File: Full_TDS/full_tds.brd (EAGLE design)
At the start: 69.5 x 52.1 mm, 66 parts, among them IC1 MCP1702, Q5 8MHz, SW1 MAIN, SW2 PI, SW3 SENSOR, U2 FT232RLSSOP, U3 ADXL345PATRICK, U4 MPL3115A2LGA8, U5 ATMEGA328P_TQFP

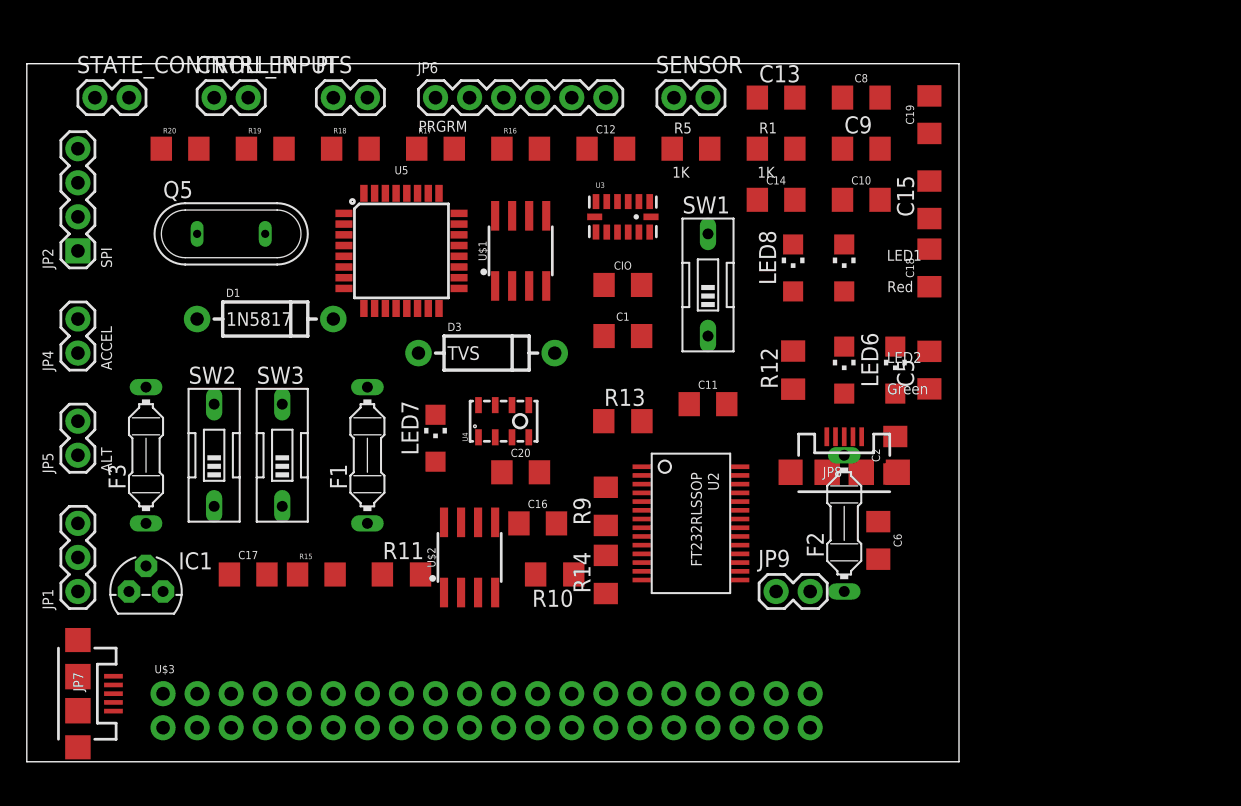
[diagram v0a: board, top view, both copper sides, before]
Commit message: Some schematic adjustments and board progress
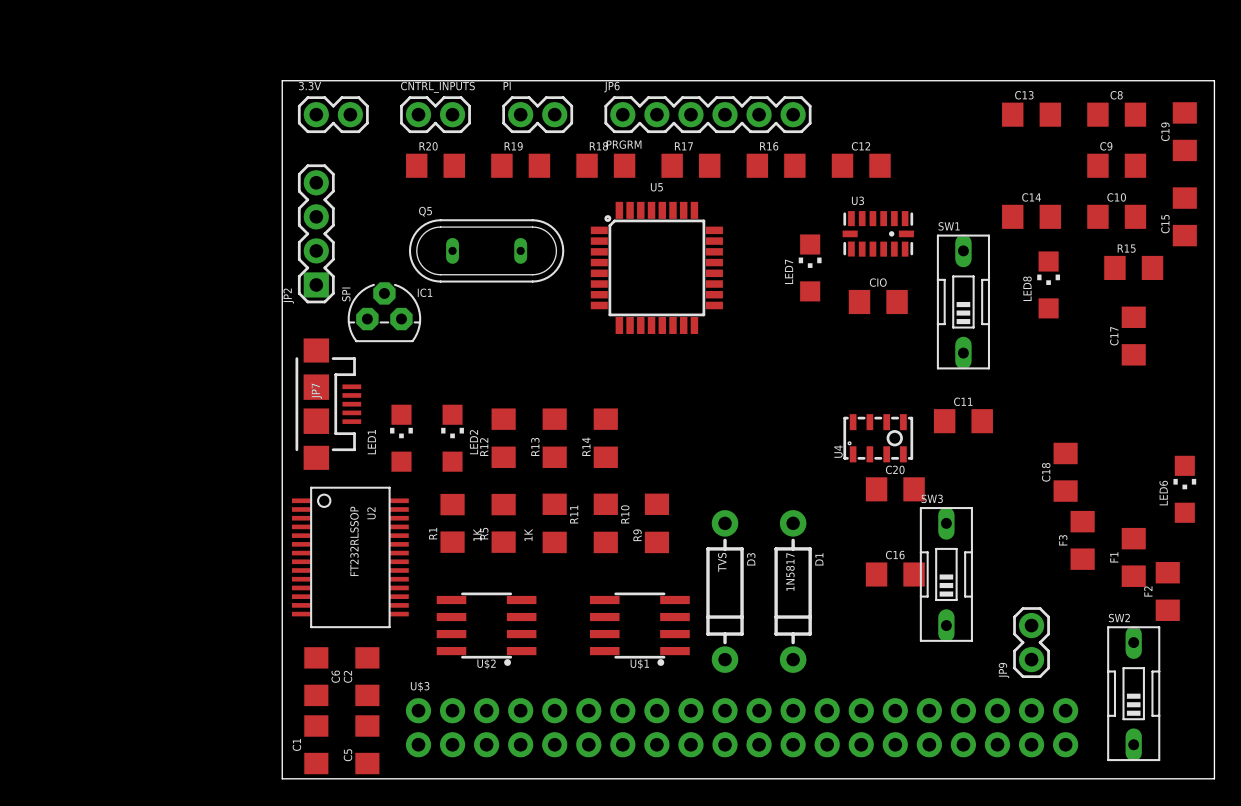
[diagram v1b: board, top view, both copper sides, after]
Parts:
- removed JP1: GPIO, SparkFun-Connectors:1X03
- removed JP4: ACCEL, SparkFun-Connectors:1X02
- removed JP5: ALT, SparkFun-Connectors:1X02
- removed JP8: USB-MICROB, SparkFun-Connectors:USB-MICROB
- removed SENSOR, STATE_CONTROLLER: (no value), SparkFun-Connectors:1X02
- added 3.3V: (no value), SparkFun-Connectors:1X02
- F1, F2, F3: device fuse:PICOFUSE -> SparkFun-Fuses:1206
- moved SW2 70.8 mm to (78.7, 8.89)
- moved F3 70.1 mm to (74.9, 20.3)
- moved C17 68.4 mm to (78.7, 35.6), turned to 90 degrees
- moved R15 65.1 mm to (78.7, 40.6)
- moved F1 57.7 mm to (78.7, 19.1)
- moved C5 50.4 mm to (21.6, 5.08)
- moved SW3 50.3 mm to (64.8, 17.8)
- moved D1 44.3 mm to (53.3, 16.5), turned to 270 degrees
- moved C6 43.1 mm to (17.8, 10.2)
- moved C2 42.7 mm to (21.6, 10.2)
- moved C1 38.1 mm to (17.8, 5.08), turned to 90 degrees
- moved R1 36.9 mm to (27.9, 21.6), turned to 90 degrees
- moved LED1 35.4 mm to (24.1, 27.9)
- moved R5 31.2 mm to (31.8, 21.6), turned to 90 degrees
- moved LED7 30.7 mm to (54.6, 40.6)
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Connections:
- removed net USB_D+: JP8.D+, U2.15
- removed net USB_D-: JP8.D-, U2.16
- removed net VBUS: C2.1, C5.1, C6.2, JP8.VBUS, U2.20
- new net D+: JP7.D+, U2.15
- new net D-: JP7.D-, U2.16
- net 3.3V: now also 3.3V.1; no longer STATE_CONTROLLER.1
- net 5V_RAW: now also C2.1, C5.1, C6.2, U2.20
- net ACCEL_INT1: no longer JP4.1
- net ACCEL_INT2: no longer JP4.2
- net ALT_INT1: no longer JP5.1
- net ALT_INT2: no longer JP5.2
- net GND-ISO: now also 3.3V.2; no longer JP8.GND, JP8.MT1, JP8.MT2, SENSOR.2, STATE_CONTROLLER.2
- net INT0: no longer JP1.1
- net INT1: no longer JP1.2
- net IO4: no longer JP1.3
- net SENSOR_POWER: no longer SENSOR.1

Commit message: Board possibly done, need more checking
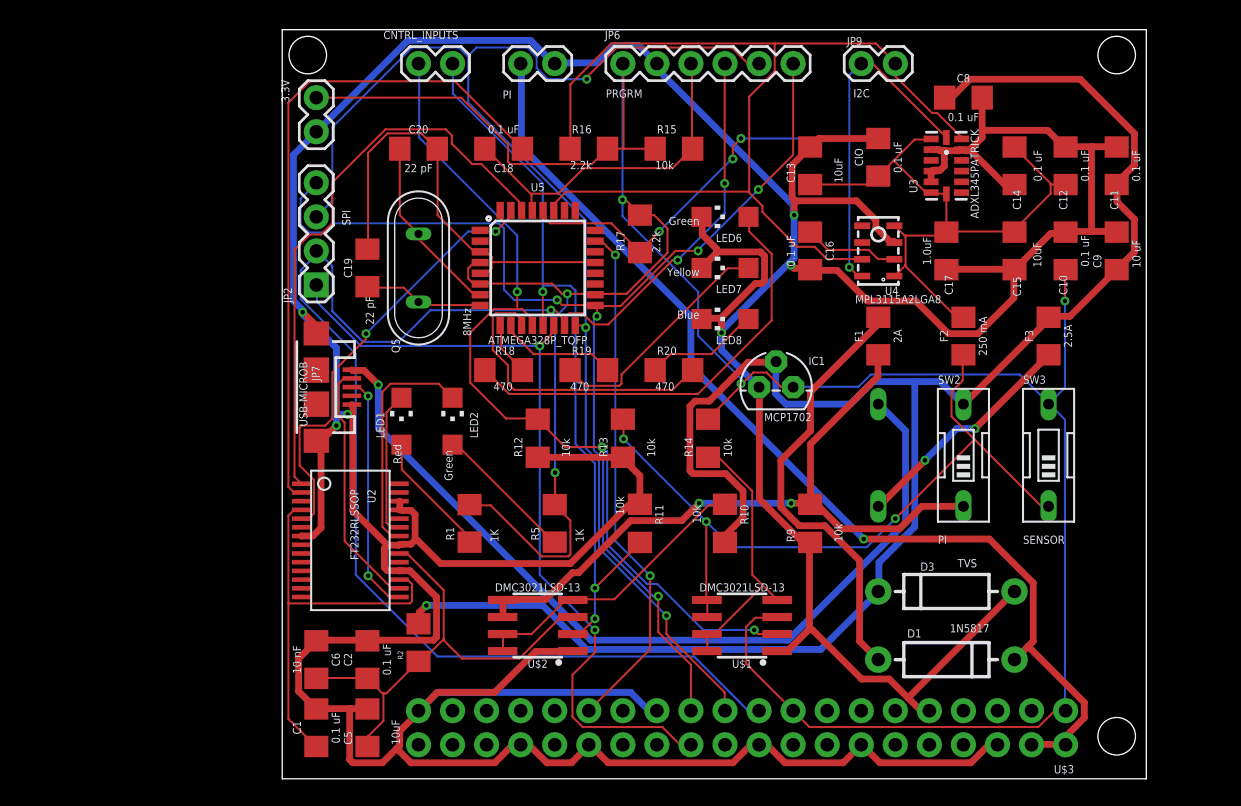
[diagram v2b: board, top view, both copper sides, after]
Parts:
- added R2: 0, SparkFun-Resistors:1206
- moved C19 61.8 mm to (21.6, 40.6)
- moved C18 48.4 mm to (31.8, 49.5), turned to 180 degrees
- moved U$3 48.3 mm to (73.7, 7.62), turned to 180 degrees
- moved JP9 45.6 mm to (61.0, 55.9), turned to 180 degrees
- moved C20 43.7 mm to (25.4, 49.5)
- moved LED6 39.9 mm to (48.3, 44.5), turned to 90 degrees
- moved R15 35.4 mm to (44.5, 49.5)
- moved IC1 29.6 mm to (52.1, 31.8)
- moved F1 25.2 mm to (59.7, 35.6)
- moved C16 25.0 mm to (54.6, 41.9), turned to 270 degrees
- moved F2 24.4 mm to (66.0, 35.6)
- moved LED8 24.3 mm to (48.3, 36.8), turned to 90 degrees
- moved R20 23.4 mm to (44.5, 33.0)
- moved C11 22.2 mm to (77.5, 48.3), turned to 90 degrees
- moved SW2 21.8 mm to (66.0, 26.7)
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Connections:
- new net FT232_VCC: C2.1, C5.1, C6.2, R2.1, U$2.3, U2.20
- net 5V: now also R2.2; no longer U$2.3, U$3.4
- net 5V_RAW: no longer C2.1, C5.1, C6.2, U2.20
- net PI_5V: now also U$3.4
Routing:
- net GND-ISO: track 0.00 -> 419.8 mm, vias 0 -> 6
- net 3.3V: track 0.00 -> 211.1 mm, vias 0 -> 5
- net 5V: track 0.00 -> 138.8 mm, vias 0 -> 1
- net MOSI: track 0.00 -> 113.3 mm, vias 0 -> 3
- net MISO: track 0.00 -> 102.6 mm, vias 0 -> 3
- net SCLK: track 0.00 -> 91.2 mm, vias 0 -> 5
- net PI_5V: track 0.00 -> 78.6 mm, vias 0 -> 1
- net SDA: track 0.00 -> 77.0 mm
- net SENSOR_PWR_CNTRL: track 0.00 -> 66.0 mm, vias 0 -> 3
- net 5V_RAW: track 0.00 -> 64.9 mm, vias 0 -> 1
- net SS: track 0.00 -> 61.0 mm, vias 0 -> 2
- net PI_PWR_CNTRL: track 0.00 -> 56.9 mm, vias 0 -> 3
- net N$6: track 0.00 -> 56.5 mm, vias 0 -> 3
- net SCL: track 0.00 -> 54.0 mm, vias 0 -> 4
- net N$3: track 0.00 -> 53.3 mm, vias 0 -> 2
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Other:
- board size 69.5 x 52.1 mm -> 64.4 x 55.9 mm
